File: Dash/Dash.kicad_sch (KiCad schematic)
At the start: 45 parts, among them CN1 NUCLEO-L432KC, J1 40 pin ZIF FPC Connector, J2 Nanofit Connector, U1 LF33_TO220, U2 LM7805_TO220, U3 BT817Q, U5 ISO1050DUB, U6 MCP2515-I/SO, U8 LM7809_TO220

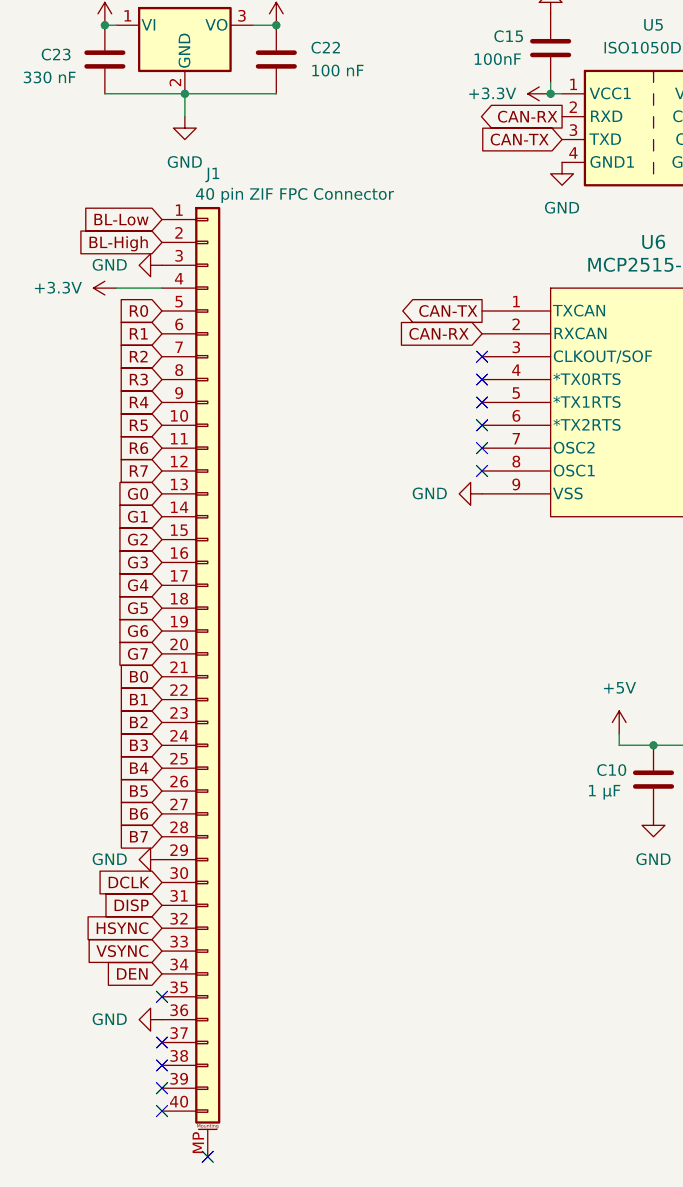
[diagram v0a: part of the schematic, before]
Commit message: Updated ribbon cable footprint and added pcb text to Dash board
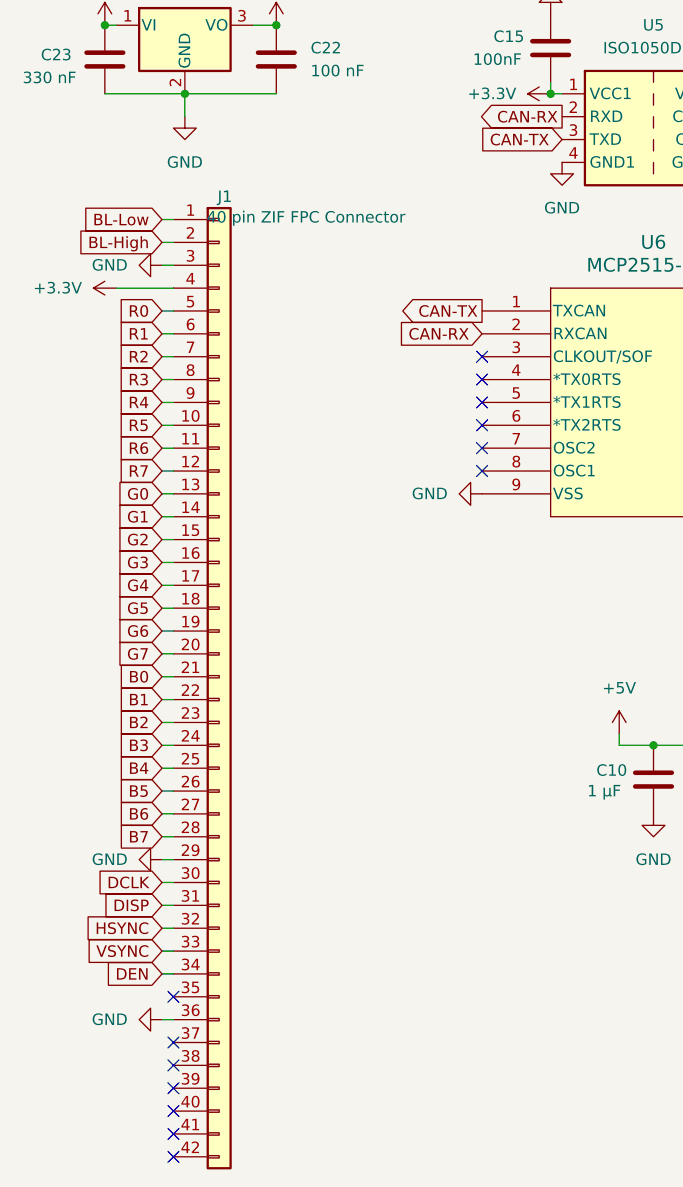
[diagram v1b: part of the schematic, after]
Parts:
- J1: footprint Connector_FFC-FPC:TE_4-1734839-0_1x40-1MP_P0.5mm_Horizontal -> FS_3_Global_Footprint_Library:CONN_F32D-1A7Y1-21040_AMP; symbol Connector_Generic_MountingPin:Conn_01x40_MountingPin -> Connector_Generic:Conn_01x42
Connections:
- no-connect marks 47 -> 48
